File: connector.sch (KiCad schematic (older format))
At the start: 1 part

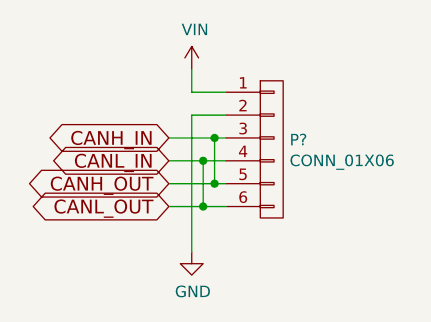
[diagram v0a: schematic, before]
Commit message: .
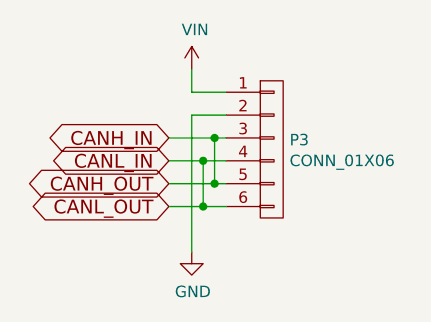
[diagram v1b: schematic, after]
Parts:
- gave numbers to parts that had none: 1
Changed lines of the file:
@@
 $EndDescr
 $Comp
-L CONN_01X06 P?
+L CONN_01X06 P3
 U 1 1 57AF467D
 P 3400 4150
-F 0 "P?" H 3478 4191 50  0000 L CNN
+F 0 "P3" H 3478 4191 50  0000 L CNN
 F 1 "CONN_01X06" H 3478 4100 50  0000 L CNN
-F 2 "" H 3400 4150 50  0000 C CNN
+F 2 "" H 3400 4150 50  0001 C CNN
 F 3 "" H 3400 4150 50  0000 C CNN
 	1    3400 4150
@@
 $EndComp
 $Comp
-L VIN #PWR?
+L VIN #PWR052
 U 1 1 57AF4ABC
 P 3050 3800
-F 0 "#PWR?" H 3050 3650 50  0001 C CNN
+F 0 "#PWR052" H 3050 3650 50  0001 C CNN
 F 1 "VIN" H 3065 3973 50  0000 C CNN
 F 2 "" H 3050 3800 60  0000 C CNN
@@
 	3050 3900 3050 3800
 $Comp
-L GND #PWR?
+L GND #PWR053
 U 1 1 57AF4B0E
 P 3050 4600
-F 0 "#PWR?" H 3050 4350 50  0001 C CNN
+F 0 "#PWR053" H 3050 4350 50  0001 C CNN
 F 1 "GND" H 3055 4427 50  0000 C CNN
 F 2 "" H 3050 4600 50  0000 C CNN

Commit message: Reset circuit, minor changes
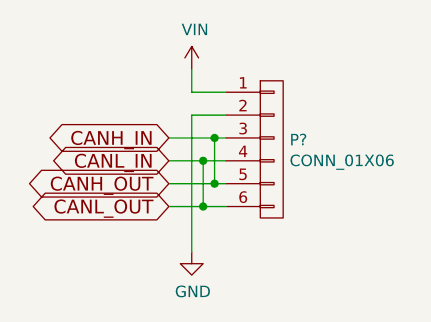
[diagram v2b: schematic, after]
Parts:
- renumbered P3 to P?
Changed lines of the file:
@@
 $EndDescr
 $Comp
-L CONN_01X06 P3
+L CONN_01X06 P?
 U 1 1 57AF467D
 P 3400 4150
-F 0 "P3" H 3478 4191 50  0000 L CNN
+F 0 "P?" H 3478 4191 50  0000 L CNN
 F 1 "CONN_01X06" H 3478 4100 50  0000 L CNN
 F 2 "" H 3400 4150 50  0001 C CNN
@@
 $EndComp
 $Comp
-L VIN #PWR052
+L VIN #PWR?
 U 1 1 57AF4ABC
 P 3050 3800
-F 0 "#PWR052" H 3050 3650 50  0001 C CNN
+F 0 "#PWR?" H 3050 3650 50  0001 C CNN
 F 1 "VIN" H 3065 3973 50  0000 C CNN
 F 2 "" H 3050 3800 60  0000 C CNN
@@
 	3050 3900 3050 3800
 $Comp
-L GND #PWR053
+L GND #PWR?
 U 1 1 57AF4B0E
 P 3050 4600
-F 0 "#PWR053" H 3050 4350 50  0001 C CNN
+F 0 "#PWR?" H 3050 4350 50  0001 C CNN
 F 1 "GND" H 3055 4427 50  0000 C CNN
 F 2 "" H 3050 4600 50  0000 C CNN
